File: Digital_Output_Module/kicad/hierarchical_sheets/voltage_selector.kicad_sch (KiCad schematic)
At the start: 1 part, among them SW1 SW_DP3T

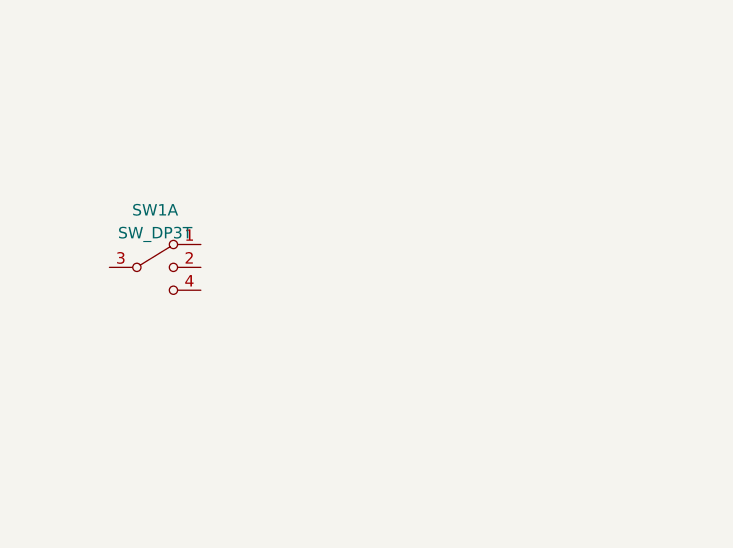
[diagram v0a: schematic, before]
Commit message: finished voltage selector switch
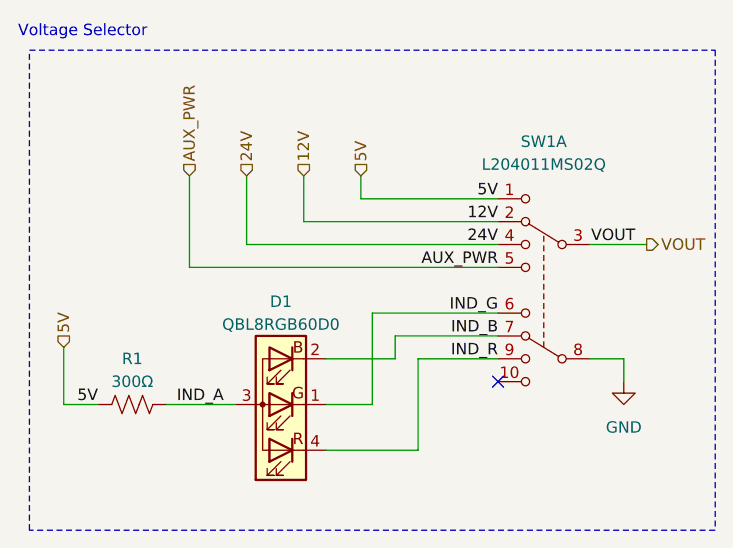
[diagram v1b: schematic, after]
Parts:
- removed SW1: SW_DP3T, symbol Switch:SW_DP3T
- added D1: QBL8RGB60D0, LED_THT:LED_D5.0mm-4_RGB, symbol Device:LED_GBAR
- added R1: 300Ω, Resistor_SMD:R_0603_1608Metric, symbol Device:R_US
- added SW1: L204011MS02Q, symbol L204011MS02Q:L204011MS02Q
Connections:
- new net 12V: SW1.2
- new net 24V: SW1.4
- new net 5V: R1.1, SW1.1
- new net AUX_PWR: SW1.5
- new net GND: SW1.8
- new net IND_A: D1.3 (A), R1.2
- new net IND_B: D1.2 (BK), SW1.7
- new net IND_G: D1.1 (GK), SW1.6
- new net IND_R: D1.4 (RK), SW1.9
- new net VOUT: SW1.3
- no-connect marks 0 -> 1
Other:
- note added: "Voltage Selector"
- company: (none) -> Missouri S&T Rocket Design Team
- title: (none) -> Voltage Selector
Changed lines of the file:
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@@
 (kicad_sch (version 20230121) (generator eeschema)
-  (paper "A4")
-  (symbol (lib_id "Switch:SW_DP3T") (at 114.3 95.25 0) (unit 1)
+  (paper "USLetter")
+  (title_block
+    (title "Voltage Selector")
+    (date "2023-03-28")
+    (rev "1")
+    (company "Missouri S&T Rocket Design Team")
+    (comment 1 "Seth Sievers")
+  )
+  (no_connect (at 152.4 107.95))
+  (wire (pts (xy 162.56 105.41) (xy 166.37 105.41))
+    (stroke (width 0) (type default))
+  )
+  (wire (pts (xy 118.11 95.25) (xy 152.4 95.25))
+    (stroke (width 0) (type default))
+  )
+  (wire (pts (xy 124.46 92.71) (xy 152.4 92.71))
+    (stroke (width 0) (type default))
+  )
+  (wire (pts (xy 104.14 110.49) (xy 107.95 110.49))
+    (stroke (width 0) (type default))
+  )
+  (wire (pts (xy 138.43 110.49) (xy 138.43 100.33))
+    (stroke (width 0) (type default))
+  )
+  (wire (pts (xy 133.35 105.41) (xy 140.97 105.41))
+    (stroke (width 0) (type default))
+  )
+  (wire (pts (xy 133.35 110.49) (xy 138.43 110.49))
+    (stroke (width 0) (type default))
+  )
+  (wire (pts (xy 138.43 100.33) (xy 152.4 100.33))
+    (stroke (width 0) (type default))
+  )
+  (wire (pts (xy 130.81 90.17) (xy 130.81 85.09))
+    (stroke (width 0) (type default))
+  )
+  (wire (pts (xy 137.16 87.63) (xy 152.4 87.63))
+    (stroke (width 0) (type default))
+  )
+  (wire (pts (xy 162.56 92.71) (xy 168.91 92.71))
+    (stroke (width 0) (type default))
+  )
+  (wire (pts (xy 143.51 115.57) (xy 143.51 105.41))
+    (stroke (width 0) (type default))
+  )
+  (wire (pts (xy 140.97 105.41) (xy 140.97 102.87))
+    (stroke (width 0) (type default))
+  )
+  (wire (pts (xy 137.16 85.09) (xy 137.16 87.63))
+    (stroke (width 0) (type default))
+  )
+  (wire (pts (xy 104.14 104.14) (xy 104.14 110.49))
+    (stroke (width 0) (type default))
+  )
+  (wire (pts (xy 166.37 105.41) (xy 166.37 107.95))
+    (stroke (width 0) (type default))
+  )
+  (wire (pts (xy 143.51 105.41) (xy 152.4 105.41))
+    (stroke (width 0) (type default))
+  )
+  (wire (pts (xy 133.35 115.57) (xy 143.51 115.57))
+    (stroke (width 0) (type default))
+  )
+  (wire (pts (xy 115.57 110.49) (xy 123.19 110.49))
+    (stroke (width 0) (type default))
+  )
+  (wire (pts (xy 130.81 90.17) (xy 152.4 90.17))
+    (stroke (width 0) (type default))
+  )
+  (wire (pts (xy 124.46 92.71) (xy 124.46 85.09))
+    (stroke (width 0) (type default))
+  )
+  (wire (pts (xy 118.11 95.25) (xy 118.11 85.09))
+    (stroke (width 0) (type default))
+  )
+  (wire (pts (xy 140.97 102.87) (xy 152.4 102.87))
+    (stroke (width 0) (type default))
+  )
+  (rectangle (start 100.33 71.12) (end 176.53 124.46)
+    (stroke (width 0) (type dash))
+    (fill (type none))
+  )
+  (text "Voltage Selector" (at 99.06 69.85 0)
+    (effects (font (size 1.27 1.27)) (justify left bottom))
+  )
+  (label "5V" (at 107.95 110.49 180) (fields_autoplaced)
+    (effects (font (size 1.27 1.27)) (justify right bottom))
+  )
+  (label "5V" (at 152.4 87.63 180) (fields_autoplaced)
+    (effects (font (size 1.27 1.27)) (justify right bottom))
+  )
+  (label "12V" (at 152.4 90.17 180) (fields_autoplaced)
+    (effects (font (size 1.27 1.27)) (justify right bottom))
+  )
+  (label "IND_A" (at 121.92 110.49 180) (fields_autoplaced)
+    (effects (font (size 1.27 1.27)) (justify right bottom))
+  )
+  (label "VOUT" (at 167.64 92.71 180) (fields_autoplaced)
+    (effects (font (size 1.27 1.27)) (justify right bottom))
+  )
+  (label "IND_B" (at 152.4 102.87 180) (fields_autoplaced)
+    (effects (font (size 1.27 1.27)) (justify right bottom))
+  )
+  (label "24V" (at 152.4 92.71 180) (fields_autoplaced)
+    (effects (font (size 1.27 1.27)) (justify right bottom))
+  )
+  (label "IND_R" (at 152.4 105.41 180) (fields_autoplaced)
+    (effects (font (size 1.27 1.27)) (justify right bottom))
+  )
+  (label "AUX_PWR" (at 152.4 95.25 180) (fields_autoplaced)
+    (effects (font (size 1.27 1.27)) (justify right bottom))
+  )
+  (label "IND_G" (at 152.4 100.33 180) (fields_autoplaced)
+    (effects (font (size 1.27 1.27)) (justify right bottom))
+  )
+  (hierarchical_label "5V" (shape input) (at 104.14 104.14 90) (fields_autoplaced)
+    (effects (font (size 1.27 1.27)) (justify left))
+  )
+  (hierarchical_label "VOUT" (shape output) (at 168.91 92.71 0) (fields_autoplaced)
+    (effects (font (size 1.27 1.27)) (justify left))
+  )
+  (hierarchical_label "AUX_PWR" (shape input) (at 118.11 85.09 90) (fields_autoplaced)
+    (effects (font (size 1.27 1.27)) (justify left))
+  )
+  (hierarchical_label "12V" (shape input) (at 130.81 85.09 90) (fields_autoplaced)
+    (effects (font (size 1.27 1.27)) (justify left))
+  )
+  (hierarchical_label "24V" (shape input) (at 124.46 85.09 90) (fields_autoplaced)
+    (effects (font (size 1.27 1.27)) (justify left))
+  )
+  (hierarchical_label "5V" (shape input) (at 137.16 85.09 90) (fields_autoplaced)
+    (effects (font (size 1.27 1.27)) (justify left))
+  )
+  (symbol (lib_id "Device:R_US") (at 111.76 110.49 90) (unit 1)
     (in_bom yes) (on_board yes) (dnp no) (fields_autoplaced)
-    (property "Reference" "SW1" (at 114.3 88.9 0)
-      (effects (font (size 1.27 1.27)))
-    )
-    (property "Value" "SW_DP3T" (at 114.3 91.44 0)
-      (effects (font (size 1.27 1.27)))
-    )
-    (property "Footprint" "" (at 98.425 90.805 0)
-      (effects (font (size 1.27 1.27)) hide)
-    )
-    (property "Datasheet" "~" (at 98.425 90.805 0)
-      (effects (font (size 1.27 1.27)) hide)
-    )
-    (pin "1")
+    (property "Reference" "R1" (at 111.76 105.41 90)
+      (effects (font (size 1.27 1.27)))
+    )
+    (property "Value" "300Ω" (at 111.76 107.95 90)
+      (effects (font (size 1.27 1.27)))
+    )
+    (property "Footprint" "Resistor_SMD:R_0603_1608Metric" (at 112.014 109.474 90)
+      (effects (font (size 1.27 1.27)) hide)
+    )
+    (property "Datasheet" "~" (at 111.76 110.49 0)
+      (effects (font (size 1.27 1.27)) hide)
+    )
+    (pin "1")
+    (pin "2")
+    (instances
+      (project "digital_output_module"
+        (path "/b62c2f25-5357-4427-9763-8fa7314ae7c3/8e375fcd-78a4-44e3-b278-544631cdf948"
+          (reference "R1") (unit 1)
+        )
+      )
+    )
+  )
+  (symbol (lib_id "power:GND") (at 166.37 107.95 0) (unit 1)
+    (in_bom yes) (on_board yes) (dnp no) (fields_autoplaced)
+    (property "Reference" "#PWR05" (at 166.37 114.3 0)
+      (effects (font (size 1.27 1.27)) hide)
+    )
+    (property "Value" "GND" (at 166.37 113.03 0)
+      (effects (font (size 1.27 1.27)))
+    )
+    (property "Footprint" "" (at 166.37 107.95 0)
+      (effects (font (size 1.27 1.27)) hide)
+    )
+    (property "Datasheet" "" (at 166.37 107.95 0)
+      (effects (font (size 1.27 1.27)) hide)
+    )
+    (pin "1")
+    (instances
+      (project "digital_output_module"
+        (path "/b62c2f25-5357-4427-9763-8fa7314ae7c3/8e375fcd-78a4-44e3-b278-544631cdf948"
+          (reference "#PWR05") (unit 1)
+        )
+      )
+    )
+  )
+  (symbol (lib_id "Device:LED_GBAR") (at 128.27 110.49 180) (unit 1)
+    (in_bom yes) (on_board yes) (dnp no) (fields_autoplaced)
+    (property "Reference" "D1" (at 128.27 99.06 0)
+      (effects (font (size 1.27 1.27)))
+    )
+    (property "Value" "QBL8RGB60D0" (at 128.27 101.6 0)
+      (effects (font (size 1.27 1.27)))
+    )
+    (property "Footprint" "LED_THT:LED_D5.0mm-4_RGB" (at 128.27 109.22 0)
+      (effects (font (size 1.27 1.27)) hide)
+    )
+    (property "Datasheet" "https://www.qt-brightek.com/datasheet/QBL8RGB60D0-2897.pdf" (at 128.27 109.22 0)
+      (effects (font (size 1.27 1.27)) hide)
+    )
+    (property "Digikey" "https://www.digikey.com/en/products/detail/qt-brightek-qtb/QBL8RGB60D0-2897/10441184" (at 128.27 110.49 0)
+      (effects (font (size 1.27 1.27)) hide)
+    )
+    (pin "1")
+    (pin "2")
+    (pin "3")
+    (pin "4")
+    (instances
+      (project "digital_output_module"
+        (path "/b62c2f25-5357-4427-9763-8fa7314ae7c3/8e375fcd-78a4-44e3-b278-544631cdf948"
+          (reference "D1") (unit 1)
+        )
+      )
+    )
+  )
+  (symbol (lib_id "L204011MS02Q:L204011MS02Q") (at 157.48 92.71 0) (mirror y) (unit 1)
+    (in_bom yes) (on_board yes) (dnp no)
+    (property "Reference" "SW1" (at 157.48 81.28 0)
+      (effects (font (size 1.27 1.27)))
+    )
+    (property "Value" "L204011MS02Q" (at 157.48 83.82 0)
+      (effects (font (size 1.27 1.27)))
+    )
+    (property "Footprint" "" (at 173.355 88.265 0)
+      (effects (font (size 1.27 1.27)) hide)
+    )
+    (property "Datasheet" "https://www.ckswitches.com/media/1423/l.pdf" (at 157.48 86.36 0)
+      (effects (font (size 1.27 1.27)) hide)
+    )
+    (property "Digikey" "https://www.digikey.com/en/products/detail/c-k/L204011MS02Q/3753644" (at 157.48 92.71 0)
+      (effects (font (size 1.27 1.27)) hide)
+    )
+    (pin "1")
+    (pin "10")
     (pin "2")
     (pin "3")
@@
     (pin "5")
     (pin "6")
+    (pin "7")
+    (pin "8")
+    (pin "9")
+    (pin "5")
+    (pin "6")
